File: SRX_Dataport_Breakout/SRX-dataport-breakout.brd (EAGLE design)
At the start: 72.6 x 19.1 mm, 16 parts

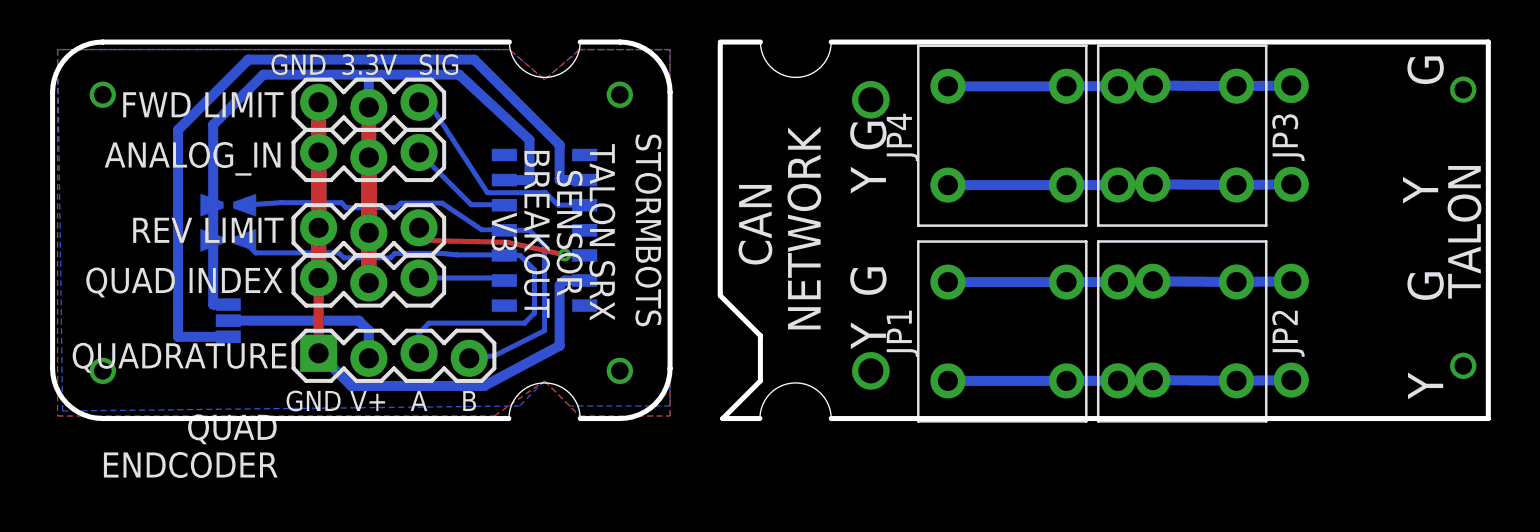
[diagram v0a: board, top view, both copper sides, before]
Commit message: Add documentation
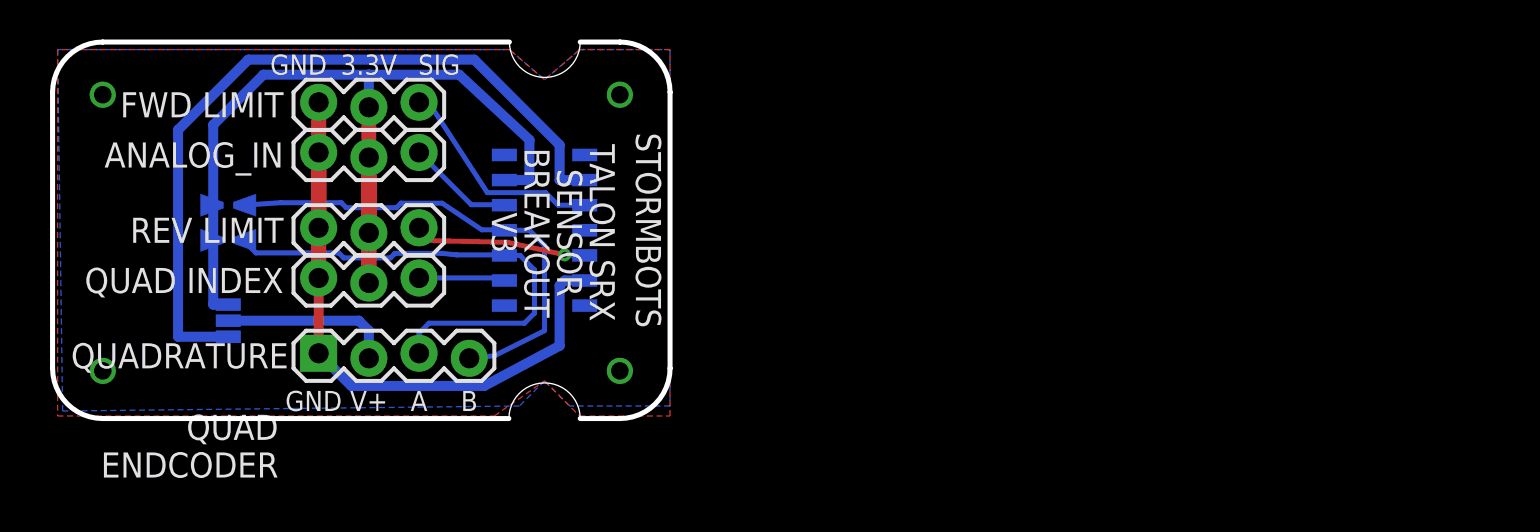
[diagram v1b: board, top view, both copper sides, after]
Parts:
- removed JP1, JP2, JP3, JP4: M022.5MM-SPRING-TERM-VERTICAL, tekdemo:1824740000-2X-VERTICAL-SPRING-TERMINAL
- removed JP5, JP6: M022.5MM-SPRING-TERM, tekdemo:1824740000-2X-STRAIGHT-SPRING-TERMINAL
- renumbered U$3 to SRX_PORT
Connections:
- removed net N$1: JP3.2A, JP3.2B, JP4.1A, JP4.1B, JP6.2A, JP6.2B
- removed net N$6: JP3.1A, JP3.1B, JP4.2A, JP4.2B, JP6.1A, JP6.1B
- removed net N$7: JP1.1A, JP1.1B, JP2.2A, JP2.2B, JP5.2A, JP5.2B
- removed net N$8: JP1.2A, JP1.2B, JP2.1A, JP2.1B, JP5.1A, JP5.1B
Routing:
- net N$8: track 17.4 -> 0.00 mm
- net N$7: track 17.4 -> 0.00 mm
- net N$6: track 17.4 -> 0.00 mm
- net N$1: track 17.4 -> 0.00 mm
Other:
- board size 72.6 x 19.1 mm -> 31.2 x 19.1 mm
- board text removed: "CAN NETWORK"
- board text removed: "G"
- board text removed: "SRX"
- board text removed: "SRX CAN BREAKOUT V3"
- board text removed: "TALON"
- board text removed: "Y"
